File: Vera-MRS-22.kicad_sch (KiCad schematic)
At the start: 18 parts, among them J4 Screw_Terminal_01x10, Q1 BC337, Q2 BC337, U2 NUCLEO-F303K8

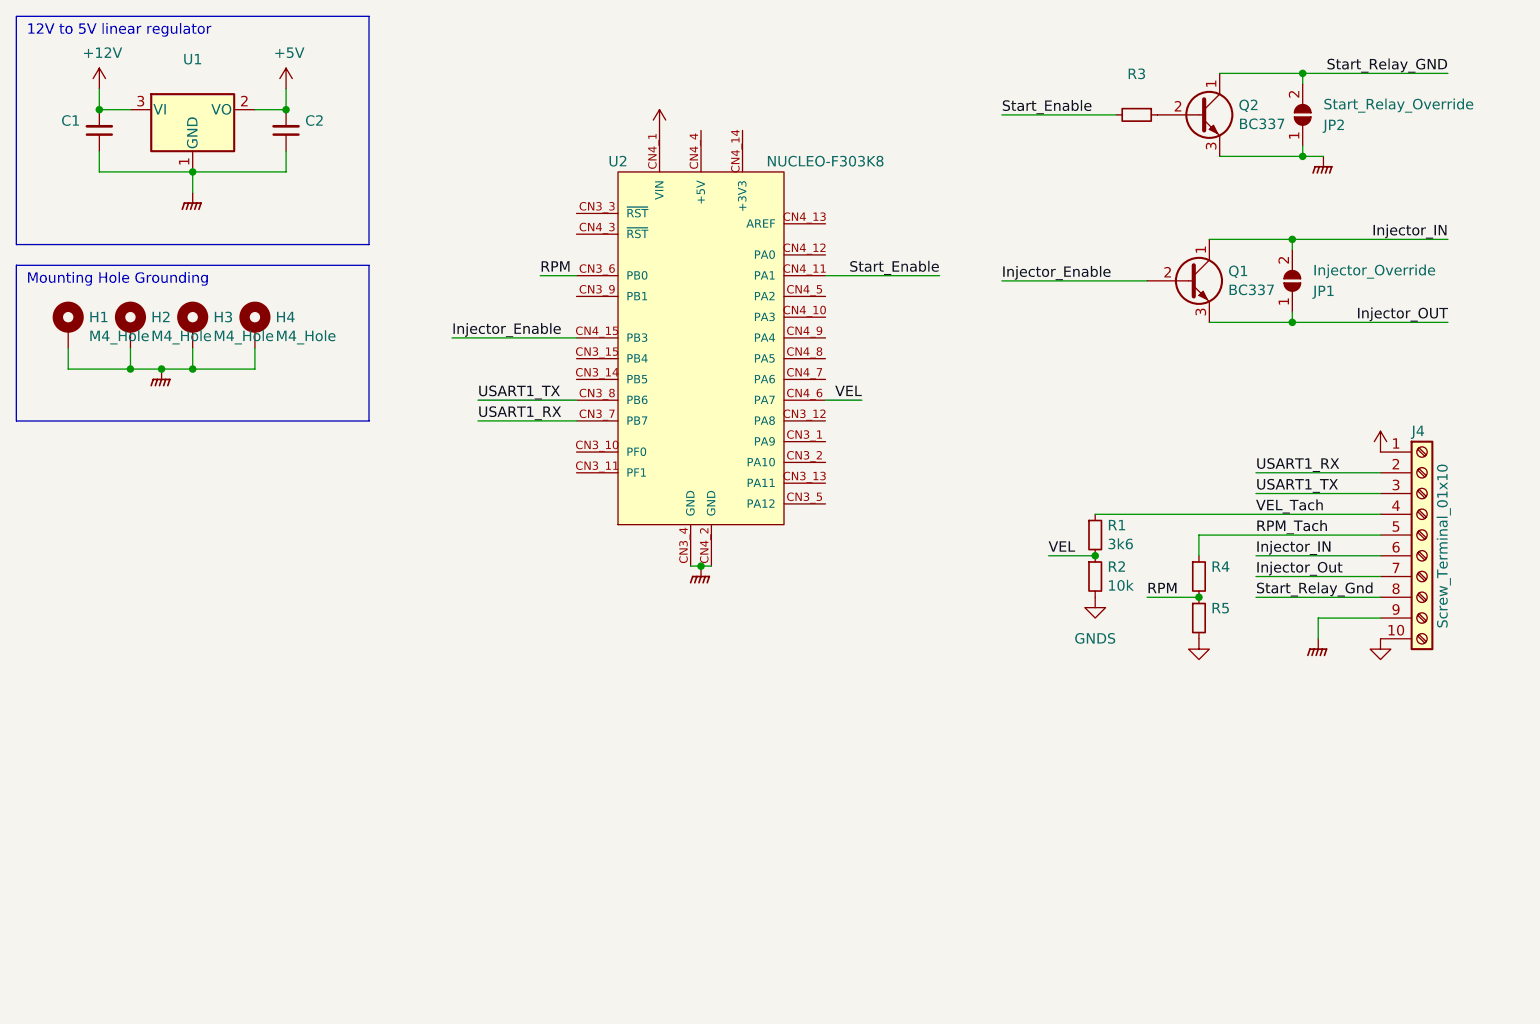
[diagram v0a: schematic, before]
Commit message: Finished RevB and sent for manufature
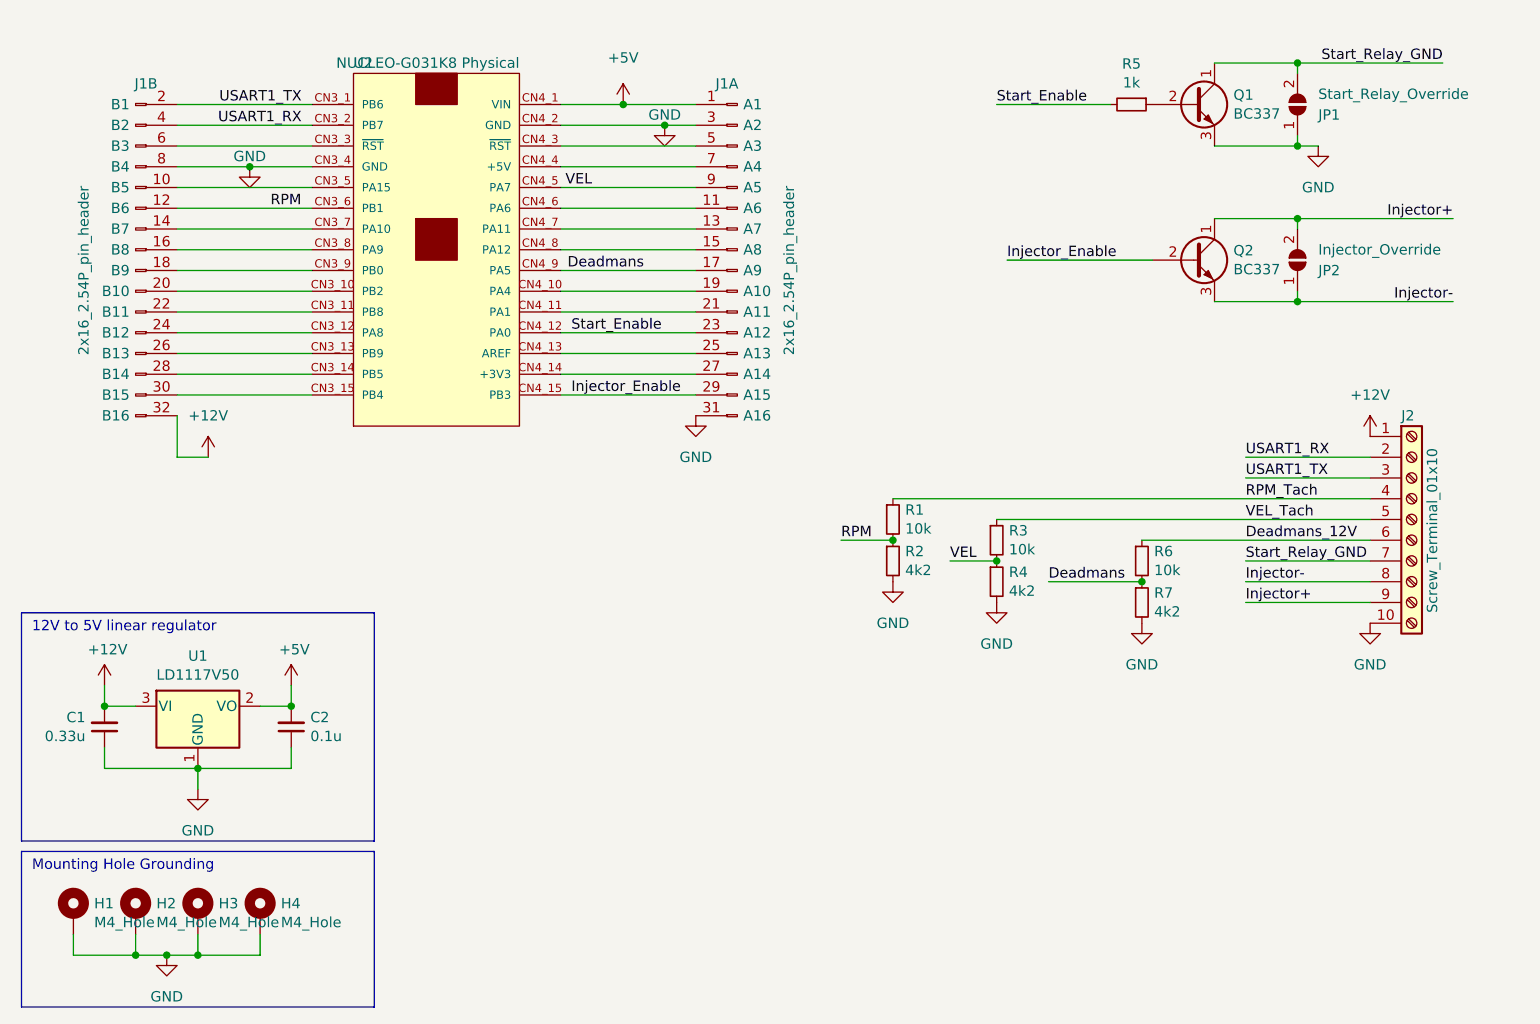
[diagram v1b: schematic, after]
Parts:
- removed U2: NUCLEO-F303K8, Vera-MRS-21:NUCLEO_32, symbol Vera-MRS-21:NUCLEO-F303K8
- added J1: 2x16_2.54P_pin_header, Connector_PinHeader_2.54mm:PinHeader_2x16_P2.54mm_Vertical, symbol Vera-MRS-21:2x16_2.54P_pin_header
- added R6: 10k, Resistor_THT:R_Axial_DIN0207_L6.3mm_D2.5mm_P10.16mm_Horizontal, symbol Motorrumsstyrning-rescue:R_Small-Device
- added R7: 4k2, Resistor_THT:R_Axial_DIN0207_L6.3mm_D2.5mm_P10.16mm_Horizontal, symbol Motorrumsstyrning-rescue:R_Small-Device
- added U2: NUCLEO-G031K8 Physical, Vera-MRS-21:NUCLEO_32, symbol Vera-MRS-21:NUCLEO-G031K8 Physical
- C1: value (none) -> 0.33u; footprint (none) -> Capacitor_SMD:C_1206_3216Metric_Pad1.33x1.80mm_HandSolder
- C2: value (none) -> 0.1u; footprint (none) -> Capacitor_SMD:C_1206_3216Metric_Pad1.33x1.80mm_HandSolder
- R1: renamed from R4; value (none) -> 10k; footprint (none) -> Resistor_THT:R_Axial_DIN0207_L6.3mm_D2.5mm_P10.16mm_Horizontal
- R2: renamed from R5; value (none) -> 4k2; footprint (none) -> Resistor_THT:R_Axial_DIN0207_L6.3mm_D2.5mm_P10.16mm_Horizontal
- R3: renamed from R1; value 3k6 -> 10k
- R4: renamed from R2; value 10k -> 4k2
- R5: renamed from R3; value (none) -> 1k; footprint (none) -> Resistor_THT:R_Axial_DIN0207_L6.3mm_D2.5mm_P10.16mm_Horizontal
- U1: value (none) -> LD1117V50; footprint (none) -> Package_TO_SOT_THT:TO-220-3_Horizontal_TabDown
- renumbered J4 to J2, JP2 to JP1, JP1 to JP2, Q2 to Q1, Q1 to Q2
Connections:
- net GNDS is gone; now on net GND: J2.10 (Pin_10), R2.2, R4.2
- net Injector_Out is gone; now on net Start_Relay_GND: J2.7 (Pin_7)
- net Start_Relay_Gnd is gone; now on net Injector-: J2.8 (Pin_8)
- net +12V: now also J1.32 (B16)
- net +5V: now also J1.1 (A1), U2.CN4_1 (VIN)
- net Injector_Enable: now also J1.29 (A15), U2.CN4_15 (PB3)
- net RPM: now also J1.12 (B6), U2.CN3_6 (PB1)
- net RPM_Tach: now also J2.4 (Pin_4); no longer J2.5 (Pin_5)
- net Start_Enable: now also J1.23 (A12), U2.CN4_12 (PA0)
- net USART1_RX: now also J1.4 (B2), U2.CN3_2 (PB7)
- net USART1_TX: now also J1.2 (B1), U2.CN3_1 (PB6)
- net VEL: now also J1.9 (A5), U2.CN4_5 (PA7)
- net VEL_Tach: now also J2.5 (Pin_5); no longer J2.4 (Pin_4)
- net GNDPWR renamed GND
- net GND: now also J1.3 (A2), J1.31 (A16), J1.8 (B4), R7.2, U2.CN3_4 (GND), U2.CN4_2 (GND); no longer J2.9 (Pin_9)
- net Injector_IN renamed Injector+
- net Injector+: now also J2.9 (Pin_9); no longer J2.6 (Pin_6)
- net Injector_OUT renamed Injector-
- new net: J1.20 (B10), U2.CN3_10 (PB2)
- new net: J1.22 (B11), U2.CN3_11 (PB8)
- new net: J1.24 (B12), U2.CN3_12 (PA8)
- new net: J1.26 (B13), U2.CN3_13 (PB9)
- new net: J1.28 (B14), U2.CN3_14 (PB5)
- new net: J1.30 (B15), U2.CN3_15 (PB4)
- new net: J1.6 (B3), U2.CN3_3 (~{RST})
- new net: J1.10 (B5), U2.CN3_5 (PA15)
- new net: J1.14 (B7), U2.CN3_7 (PA10)
- new net: J1.16 (B8), U2.CN3_8 (PA9)
- new net: J1.18 (B9), U2.CN3_9 (PB0)
- new net: J1.19 (A10), U2.CN4_10 (PA4)
- new net: J1.21 (A11), U2.CN4_11 (PA1)
- new net: J1.25 (A13), U2.CN4_13 (AREF)
- new net: J1.27 (A14), U2.CN4_14 (+3V3)
- new net: J1.5 (A3), U2.CN4_3 (~{RST})
- new net: J1.7 (A4), U2.CN4_4 (+5V)
- new net: J1.11 (A6), U2.CN4_6 (PA6)
- new net: J1.13 (A7), U2.CN4_7 (PA11)
- new net: J1.15 (A8), U2.CN4_8 (PA12)
- new net Deadmans: J1.17 (A9), R6.2, R7.1, U2.CN4_9 (PA5)
- new net Deadmans_12V: J2.6 (Pin_6), R6.1
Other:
- moved on the sheet: C1, C2, H1, H2, H3, H4, J2, JP1, JP2, Q1, Q2, R1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
